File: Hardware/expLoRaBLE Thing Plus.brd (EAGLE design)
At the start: 22.9 x 58.4 mm, 146 parts, among them J2 CORTEX_DEBUG, J5 USB Female Type C Connector, J6 QWIIC_RIGHT_ANGLE, J8 U.FL, U1 MCP73831, U2 3.3V, U3 NM180100, U4 CH340E_MSOP10, U6 DPX202700DT-4162A1, Y1 32.768kHz

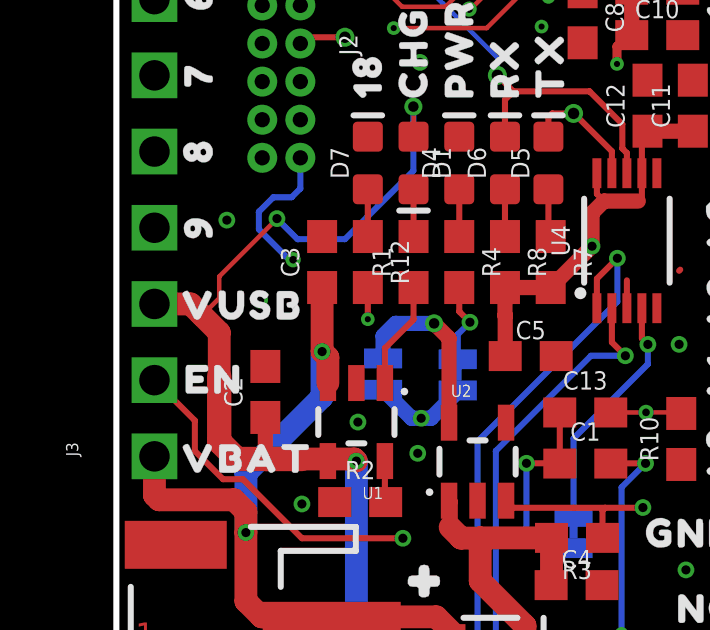
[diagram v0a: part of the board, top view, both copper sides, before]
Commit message: Actual group review changes
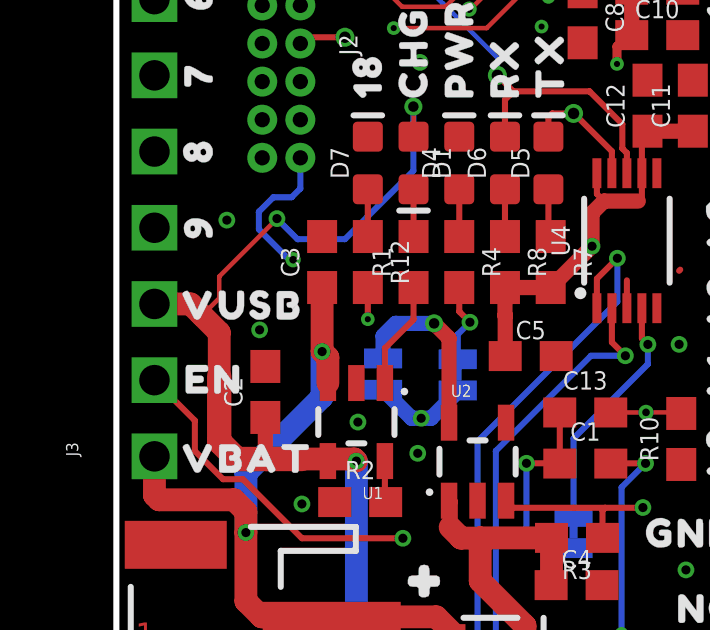
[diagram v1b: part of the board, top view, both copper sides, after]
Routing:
- net 3.3V: track 43.5 -> 44.5 mm
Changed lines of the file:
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@@
 <grid distance="0.05" unitdist="inch" unit="inch" style="lines" multiple="1" display="yes" altdistance="0.001" altunitdist="inch" altunit="inch"/>
 <layers>
-<layer number="1" name="Top" color="4" fill="1" visible="no" active="yes"/>
+<layer number="1" name="Top" color="4" fill="1" visible="yes" active="yes"/>
 <layer number="2" name="Route2" color="11" fill="3" visible="yes" active="yes"/>
 <layer number="3" name="Route3" color="17" fill="1" visible="no" active="no"/>
@@
 <layer number="13" name="Route13" color="21" fill="1" visible="no" active="no"/>
 <layer number="14" name="Route14" color="22" fill="1" visible="no" active="no"/>
-<layer number="15" name="Route15" color="13" fill="6" visible="no" active="yes"/>
-<layer number="16" name="Bottom" color="1" fill="1" visible="no" active="yes"/>
+<layer number="15" name="Route15" color="13" fill="6" visible="yes" active="yes"/>
+<layer number="16" name="Bottom" color="1" fill="1" visible="yes" active="yes"/>
 <layer number="17" name="Pads" color="2" fill="1" visible="yes" active="yes"/>
 <layer number="18" name="Vias" color="2" fill="1" visible="yes" active="yes"/>
 <layer number="19" name="Unrouted" color="6" fill="1" visible="yes" active="yes"/>
 <layer number="20" name="Dimension" color="24" fill="1" visible="yes" active="yes"/>
-<layer number="21" name="tPlace" color="16" fill="1" visible="no" active="yes"/>
-<layer number="22" name="bPlace" color="14" fill="1" visible="no" active="yes"/>
-<layer number="23" name="tOrigins" color="15" fill="1" visible="no" active="yes"/>
-<layer number="24" name="bOrigins" color="15" fill="1" visible="no" active="yes"/>
+<layer number="21" name="tPlace" color="16" fill="1" visible="yes" active="yes"/>
+<layer number="22" name="bPlace" color="14" fill="1" visible="yes" active="yes"/>
+<layer number="23" name="tOrigins" color="15" fill="1" visible="yes" active="yes"/>
+<layer number="24" name="bOrigins" color="15" fill="1" visible="yes" active="yes"/>
 <layer number="25" name="tNames" color="7" fill="1" visible="no" active="yes"/>
 <layer number="26" name="bNames" color="7" fill="1" visible="no" active="yes"/>
 <layer number="27" name="tValues" color="7" fill="1" visible="no" active="yes"/>
 <layer number="28" name="bValues" color="7" fill="1" visible="no" active="yes"/>
-<layer number="29" name="tStop" color="7" fill="3" visible="yes" active="yes"/>
+<layer number="29" name="tStop" color="7" fill="3" visible="no" active="yes"/>
 <layer number="30" name="bStop" color="7" fill="6" visible="no" active="yes"/>
 <layer number="31" name="tCream" color="7" fill="4" visible="no" active="yes"/>
@@
 <layer number="47" name="Measures" color="7" fill="1" visible="no" active="yes"/>
 <layer number="48" name="Document" color="7" fill="1" visible="no" active="yes"/>
-<layer number="49" name="Reference" color="7" fill="1" visible="no" active="yes"/>
+<layer number="49" name="Reference" color="7" fill="1" visible="yes" active="yes"/>
 <layer number="50" name="dxf" color="7" fill="1" visible="no" active="no"/>
-<layer number="51" name="tDocu" color="6" fill="1" visible="no" active="yes"/>
+<layer number="51" name="tDocu" color="6" fill="1" visible="yes" active="yes"/>
 <layer number="52" name="bDocu" color="6" fill="1" visible="no" active="yes"/>
 <layer number="53" name="tGND_GNDA" color="7" fill="9" visible="no" active="no"/>
@@
 <wire x1="14.4018" y1="39.4462" x2="14.5709" y2="39.6153" width="0.2032" layer="1"/>
 <wire x1="15.5424" y1="39.6153" x2="14.5709" y2="39.6153" width="0.2032" layer="1"/>
-<via x="4.7752" y="29.337" extent="1-16" drill="0.3048"/>
+<via x="4.7752" y="28.3464" extent="1-16" drill="0.3048"/>
 <via x="9.525" y="42.4688" extent="1-16" drill="0.2032"/>
 <via x="12.2354" y="42.4688" extent="1-16" drill="0.2032"/>
@@
 <via x="6.8834" y="42.4688" extent="1-16" drill="0.2032"/>
 <via x="3.683" y="32.004" extent="1-16" drill="0.3048"/>
-<wire x1="3.683" y1="32.004" x2="3.683" y2="30.4292" width="0.508" layer="15"/>
-<wire x1="3.683" y1="30.4292" x2="4.7752" y2="29.337" width="0.508" layer="15"/>
+<wire x1="3.683" y1="32.004" x2="3.683" y2="29.4386" width="0.508" layer="15"/>
+<wire x1="4.7752" y1="28.3464" x2="3.683" y2="29.4386" width="0.508" layer="15"/>
 <contactref element="LED" pad="2"/>
 <contactref element="ISO" pad="1"/>
